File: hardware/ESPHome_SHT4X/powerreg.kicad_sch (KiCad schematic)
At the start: 17 parts, among them SW1 SW_Push, U2 BQ25628ERYKR

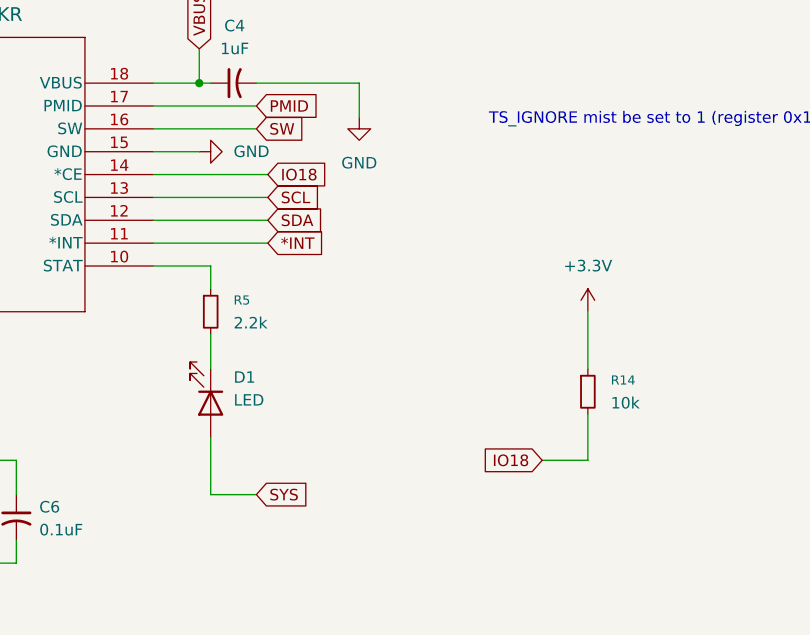
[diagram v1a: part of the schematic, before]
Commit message: Working
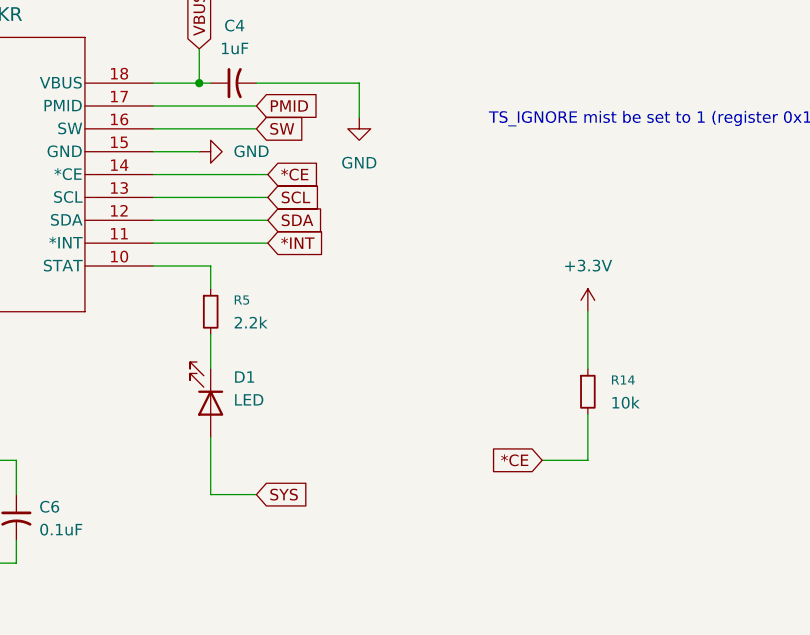
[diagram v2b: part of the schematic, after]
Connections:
- net IO18 renamed *CE
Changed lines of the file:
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@@
 		)
 	)
-	(global_label "IO18"
+	(global_label "*CE"
 		(shape input)
 		(at 198.12 119.38 180)
@@
 		)
 		(property "Intersheetrefs" "${INTERSHEET_REFS}"
-			(at 190.7805 119.38 0)
+			(at 191.7482 119.38 0)
 			(hide yes)
 			(show_name no)
@@
 		)
 	)
-	(global_label "IO18"
+	(global_label "*CE"
 		(shape input)
 		(at 167.64 87.63 0)
@@
 		)
 		(property "Intersheetrefs" "${INTERSHEET_REFS}"
-			(at 174.9795 87.63 0)
+			(at 174.0118 87.63 0)
 			(hide yes)
 			(show_name no)

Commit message: Working
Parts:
- D1, D2: footprint LED_SMD:LED_1206_3216Metric_Pad1.42x1.75mm_HandSolder -> LED_SMD:LED_0603_1608Metric_Pad1.05x0.95mm_HandSolder
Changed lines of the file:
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@@
 			)
 		)
-		(property "Footprint" "LED_SMD:LED_1206_3216Metric_Pad1.42x1.75mm_HandSolder"
+		(property "Footprint" "LED_SMD:LED_0603_1608Metric_Pad1.05x0.95mm_HandSolder"
 			(at 161.29 113.03 0)
 			(hide yes)
@@
 			)
 		)
-		(property "Footprint" "LED_SMD:LED_1206_3216Metric_Pad1.42x1.75mm_HandSolder"
+		(property "Footprint" "LED_SMD:LED_0603_1608Metric_Pad1.05x0.95mm_HandSolder"
 			(at 92.71 73.66 0)
 			(hide yes)
@@
 		)
 	)
+	(embedded_fonts no)
 )
